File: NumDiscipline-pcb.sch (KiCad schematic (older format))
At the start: 190 parts, among them J1 AVR-ISP-6, SW1 KEYSW, SW10 KEYSW, SW11 KEYSW, SW12 KEYSW, SW13 KEYSW, SW14 KEYSW, SW15 KEYSW, SW16 KEYSW, SW17 KEYSW, SW18 KEYSW, SW19 KEYSW, SW2 KEYSW, SW20 KEYSW, SW21 KEYSW, SW22 KEYSW, SW23 KEYSW, SW24 KEYSW, SW25 KEYSW, SW26 KEYSW, SW27 KEYSW, SW28 KEYSW, SW29 KEYSW, SW3 KEYSW, SW30 KEYSW, SW31 KEYSW, SW32 KEYSW, SW33 KEYSW, SW34 KEYSW, SW35 KEYSW, SW36 KEYSW, SW37 KEYSW, SW38 KEYSW, SW39 KEYSW, SW4 KEYSW, SW40 KEYSW, SW41 KEYSW, SW42 KEYSW, SW43 KEYSW, SW44 KEYSW, SW45 KEYSW, SW46 KEYSW, SW47 KEYSW, SW48 KEYSW, SW49 KEYSW, SW5 KEYSW, SW50 KEYSW, SW51 KEYSW, SW52 KEYSW, SW53 KEYSW, SW54 KEYSW, SW55 KEYSW, SW56 KEYSW, SW57 KEYSW, SW58 KEYSW, SW59 KEYSW, SW6 KEYSW, SW60 KEYSW, SW61 KEYSW, SW62 KEYSW, SW63 KEYSW, SW64 KEYSW, SW65 KEYSW, SW66 KEYSW, SW67 KEYSW, SW68 KEYSW, SW69 KEYSW, SW7 KEYSW, SW70 KEYSW, SW71 KEYSW, SW72 KEYSW, SW73 KEYSW, SW74 KEYSW, SW75 KEYSW, SW76 KEYSW, SW77 KEYSW, SW78 KEYSW, SW79 KEYSW, SW8 KEYSW, SW80 KEYSW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

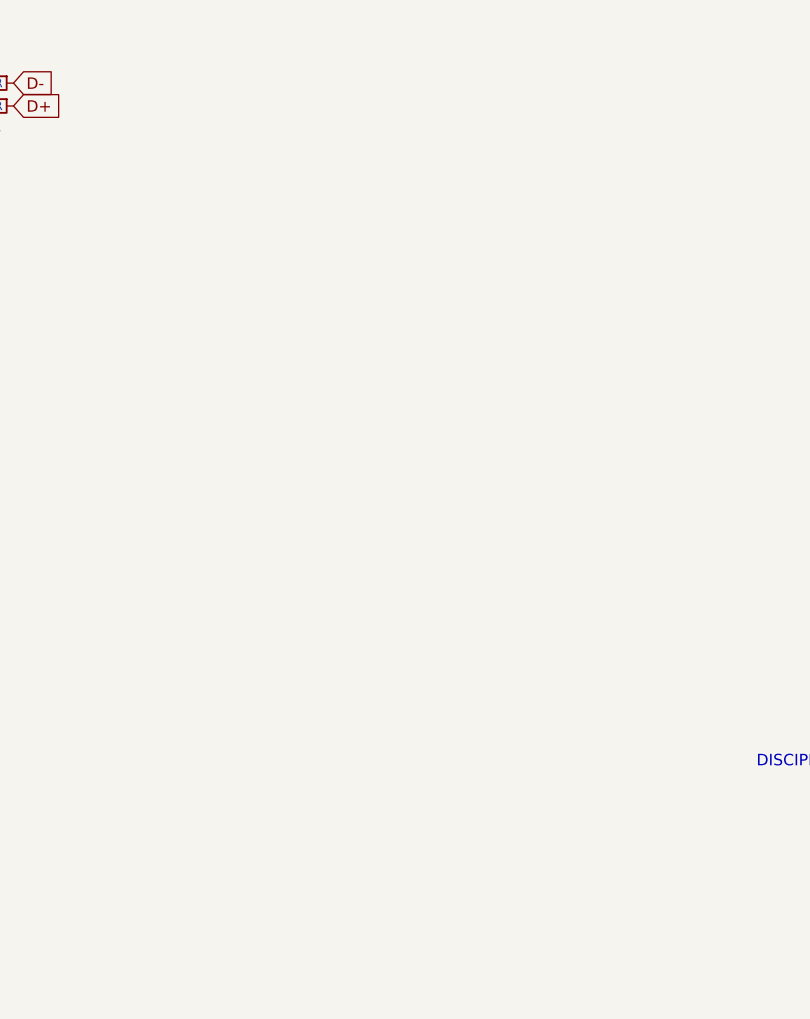
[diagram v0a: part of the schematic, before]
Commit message: add plate
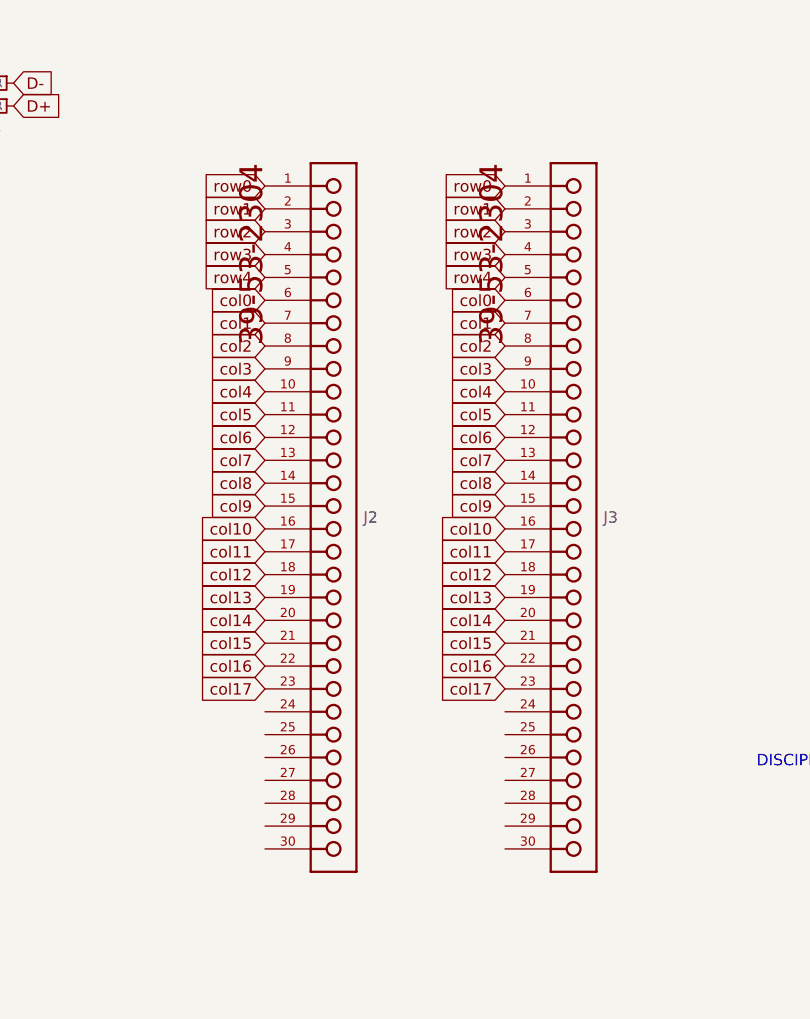
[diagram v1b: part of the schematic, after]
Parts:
- added J2, J3: MOLEX_39-53-2304, MOLEX_39-53-2304:MOLEX_39-53-2304_0, symbol MOLEX_39-53-2304:MOLEX_39-53-2304
- SW1: value KEYSW -> ESCAPE
- SW2: value KEYSW -> 1
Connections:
- net col0: now also J2.6, J3.6
- net col1: now also J2.7, J3.7
- net col10: now also J2.16, J3.16
- net col11: now also J2.17, J3.17
- net col12: now also J2.18, J3.18
- net col13: now also J2.19, J3.19
- net col14: now also J2.20, J3.20
- net col15: now also J2.21, J3.21
- net col16: now also J2.22, J3.22
- net col17: now also J2.23, J3.23
- net col2: now also J2.8, J3.8
- net col3: now also J2.9, J3.9
- net col4: now also J2.10, J3.10
- net col5: now also J2.11, J3.11
- net col6: now also J2.12, J3.12
- net col7: now also J2.13, J3.13
- net col8: now also J2.14, J3.14
- net col9: now also J2.15, J3.15
- net row0: now also J2.1, J3.1
- net row1: now also J2.2, J3.2
- net row2: now also J2.3, J3.3
- net row3: now also J2.4, J3.4
- net row4: now also J2.5, J3.5
